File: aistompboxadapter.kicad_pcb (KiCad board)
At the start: 2 copper layers, 42 x 30 mm, 24 parts, among them J1 SYNTH IN, J2 FX RETURN, J3 Synth Power, J4 FX SEND, J5 SYNTH OUT, U1 TL072

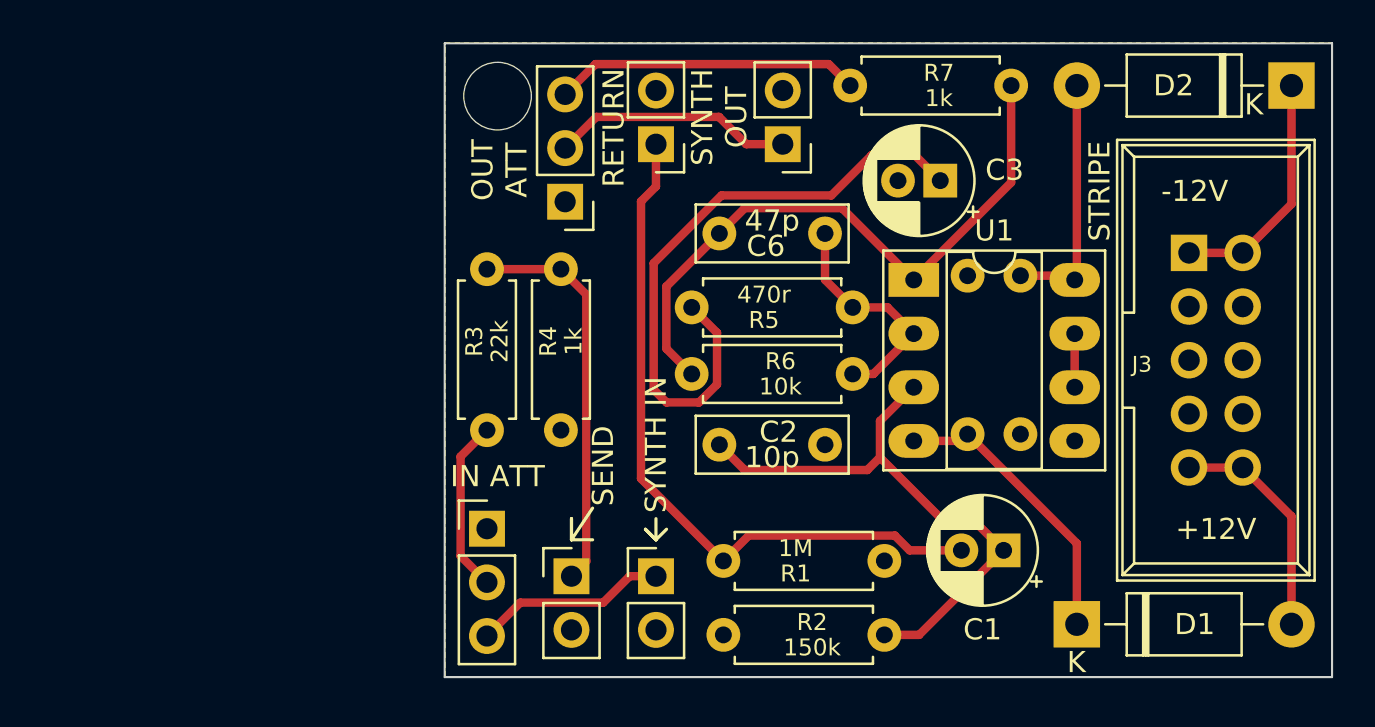
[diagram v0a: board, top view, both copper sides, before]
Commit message: smd and add fab files
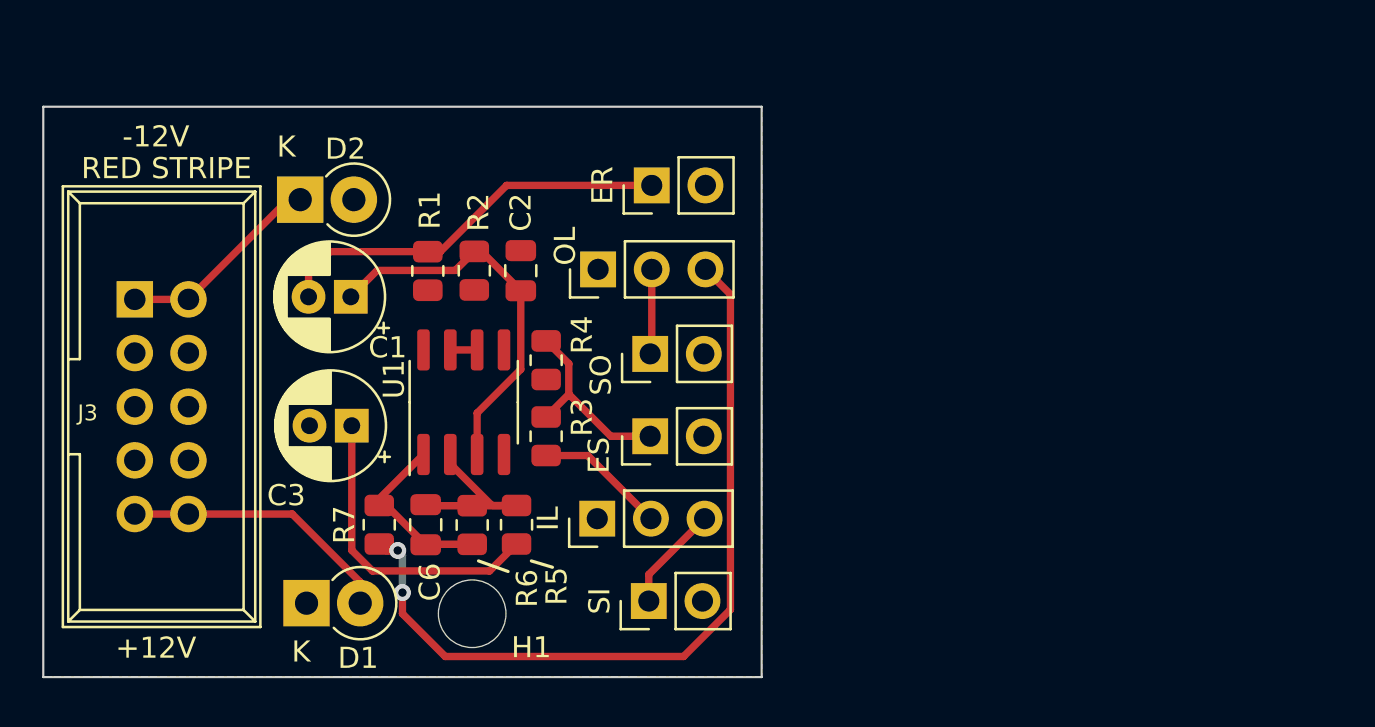
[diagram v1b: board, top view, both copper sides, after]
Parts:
- removed C4, C5: 100n, Sonosus:C_Disc_D3.0mm_W2.0mm_P2.50mm
- removed J1: SYNTH IN, Connector_PinHeader_2.54mm:PinHeader_1x02_P2.54mm_Vertical
- removed J2: FX RETURN, Connector_PinHeader_2.54mm:PinHeader_1x02_P2.54mm_Vertical
- removed J4: FX SEND, Connector_PinHeader_2.54mm:PinHeader_1x02_P2.54mm_Vertical
- removed J5: SYNTH OUT, Connector_PinHeader_2.54mm:PinHeader_1x02_P2.54mm_Vertical
- removed RV1, RV2: 100k, Connector_PinHeader_2.54mm:PinHeader_1x03_P2.54mm_Vertical
- added ER: FX RETURN, Connector_PinHeader_2.54mm:PinHeader_1x02_P2.54mm_Vertical, F.Cu at (232.8, 26.7)
- added ES: FX SEND, Connector_PinHeader_2.54mm:PinHeader_1x02_P2.54mm_Vertical, F.Cu at (232.7, 38.6)
- added IL: 100k, Connector_PinHeader_2.54mm:PinHeader_1x03_P2.54mm_Vertical, F.Cu at (230.2, 42.5)
- added OL: 100k, Connector_PinHeader_2.54mm:PinHeader_1x03_P2.54mm_Vertical, F.Cu at (230.3, 30.7)
- added SI: SI, Connector_PinHeader_2.54mm:PinHeader_1x02_P2.54mm_Vertical, F.Cu at (232.7, 46.4)
- added SO: SYNTH OUT, Connector_PinHeader_2.54mm:PinHeader_1x02_P2.54mm_Vertical, F.Cu at (232.7, 34.7)
- C2, C6: footprint Sonosus:C_Rect_L7.0mm_W2.5mm_P5.00mm -> Capacitor_SMD:C_0805_2012Metric
- D1, D2: footprint Diode_THT:D_DO-41_SOD81_P10.16mm_Horizontal -> Diode_THT:D_DO-41_SOD81_P2.54mm_Vertical_KathodeUp
- R1, R2, R3, R4, R5, R6, R7: footprint Sonosus:R_Axial_DIN0207_L6.3mm_D2.5mm_P7.62mm_Horizontal -> Resistor_SMD:R_0805_2012Metric
- U1: footprint Sonosus:DIP-8_W7.62mm_Socket_LongPads -> Package_SO:SOIC-8_3.9x4.9mm_P1.27mm
- moved J3 49.9 mm to (208.3, 32.1)
- moved D2 47.2 mm to (216.2, 27.4), turned to 0 degrees
- moved D1 36.5 mm to (216.5, 46.5)
- moved C1 33.1 mm to (218.6, 32.0)
- moved R7 30.5 mm to (219.9, 42.8), turned to 90 degrees
- moved C3 30.2 mm to (218.6, 38.1)
- moved R1 25.6 mm to (222.2, 30.8), turned to 90 degrees
- moved H1 24.5 mm to (224.3, 47.0)
- moved C6 23.4 mm to (222.1, 42.8), turned to -90 degrees
- moved U1 22.1 mm to (223.9, 37.0), turned to 90 degrees
- moved R2 20.9 mm to (224.4, 30.8), turned to 90 degrees
- moved R5 18.9 mm to (226.4, 42.8), turned to -90 degrees
- moved R6 12.6 mm to (224.3, 42.8), turned to 90 degrees
- moved C2 12.5 mm to (226.6, 30.8), turned to 90 degrees
- moved R4 3.38 mm to (227.8, 35.0)
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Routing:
- net Net-(R7-Pad1): track 14.5 -> 38.0 mm, vias 0 -> 2
- net Net-(C6-Pad2): track 30.4 -> 8.46 mm
- net Net-(C3-Pad1): track 29.9 -> 14.6 mm
- net Net-(C1-Pad2): track 33.7 -> 19.1 mm
- net +12V: track 13.8 -> 0.00 mm
- net -12V: track 11.9 -> 0.00 mm
- net Net-(RV2-Pad2): track 11.4 -> 0.00 mm
- net Net-(J4-Pad1): track 18.8 -> 9.16 mm
- net Net-(RV1-Pad3): track 9.17 -> 0.00 mm
- net Net-(C1-Pad1): track 27.3 -> 18.3 mm
- net Net-(J1-Pad1): track 0.00 -> 4.99 mm
- net Net-(J5-Pad1): track 0.00 -> 4.03 mm
- net Net-(C6-Pad1): track 11.1 -> 8.72 mm
- net Net-(D1-Pad2): track 10.9 -> 13.0 mm
- net Net-(R3-Pad1): track 8.24 -> 6.20 mm
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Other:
- board size 42 x 30 mm -> 34 x 27 mm
- board text added: "AI STOMPBOX ADAPTER PCB BY SONOSUS JAN 2021"
- board text removed: "AI SYNTHESIS STOMPBOX ADAPTER"
- board text removed: "DESIGN BY AI SYNTHESIS"
- board text removed: "IN ATT"
- board text removed: "OUT ATT"
- board text removed: "PCB BY SONOSUS JAN 2022"
- board text removed: "PCB VER. 1.0 9/1/22"
- board text removed: "RETURN"
- board text removed: "SEND"
- board text removed: "SYNTH IN"
- board text removed: "SYNTH OUT"
- board text removed: "github.com/sonosus/stompboxadapter"
